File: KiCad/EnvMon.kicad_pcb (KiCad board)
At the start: 2 copper layers, 44.5 x 37 mm, 33 parts, among them J1 USB-C, J2 DC, J3 GPIO, M1 SCD30-4pin, M2 OLED1.5-RGB, U1 LMR16006+FB, U2 FT231XQ, U3 ESP32-WROOM-32

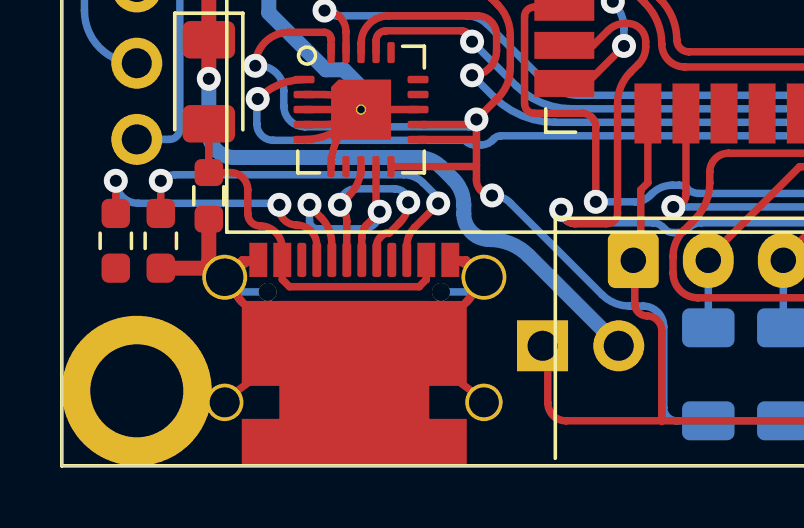
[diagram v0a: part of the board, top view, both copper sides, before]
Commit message: Notes
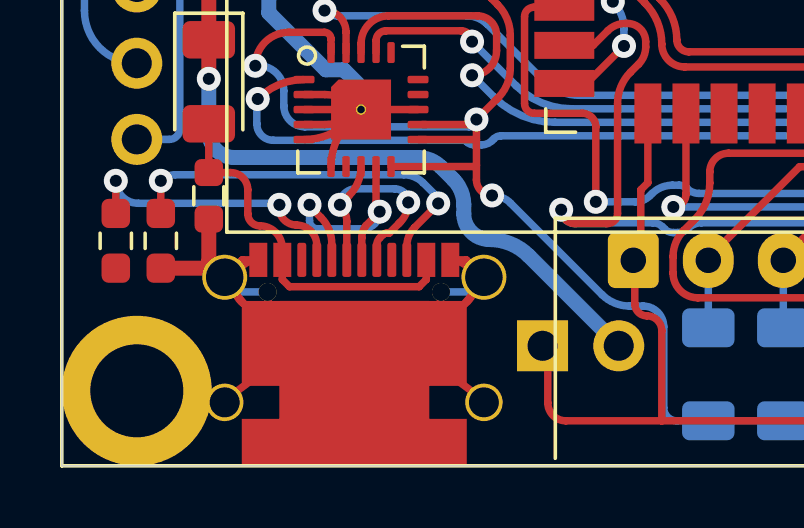
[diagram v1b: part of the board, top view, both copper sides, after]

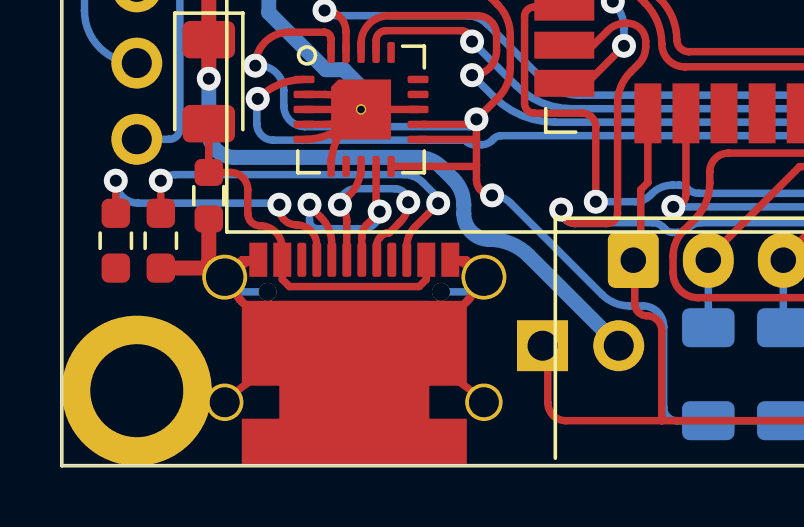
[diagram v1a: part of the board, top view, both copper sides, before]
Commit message: Resitors
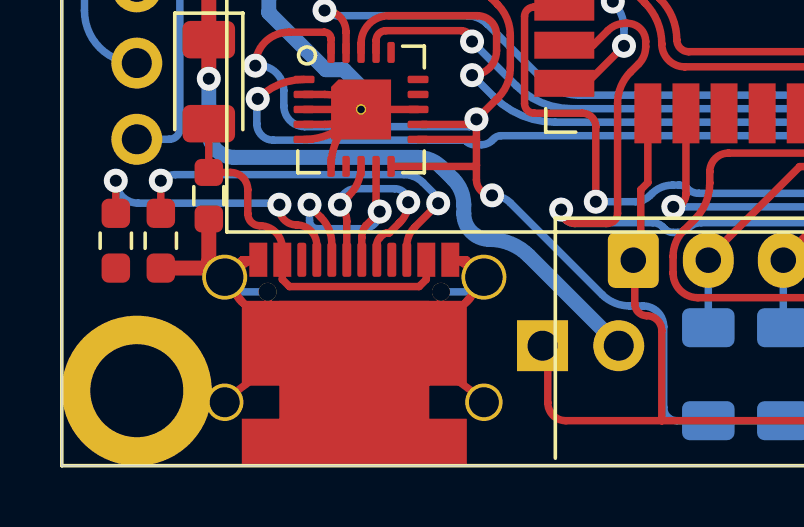
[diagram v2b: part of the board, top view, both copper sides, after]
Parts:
- R1: value 10M 1% or 0R -> 100k 1% or 0R
- R2: value 3M 1% or NF -> 30k 1% or NF
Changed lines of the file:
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@@
       (primitives
     (gr_arc (start 2.89 -3.045) (mid 0 -0.155) (end -2.89 -3.045) (width 0.25))
-    (gr_arc (start 4.294753 -3.49127) (mid -0.016568 -1.026234) (end -4.311371 -3.519937) (width 0.25))
+    (gr_arc (start 4.294753 -3.49127) (mid -0.012228 -1.026222) (end -4.307036 -3.512417) (width 0.25))
     (gr_arc (start -3.2 -2.485) (mid -4.015 -3.3) (end -3.2 -4.115) (width 0.25))
     (gr_arc (start 3.2 -4.115) (mid 4.015 -3.3) (end 3.2 -2.485) (width 0.25))
@@
       (effects (font (size 0.5 0.5) (thickness 0.08)))
     )
-    (fp_text value "10M 1% or 0R" (at 0 0 90) (layer "F.Fab")
+    (fp_text value "100k 1% or 0R" (at 0 0 90) (layer "F.Fab")
       (effects (font (size 0.4 0.4) (thickness 0.08)))
     )
@@
       (effects (font (size 0.5 0.5) (thickness 0.08)))
     )
-    (fp_text value "3M 1% or NF" (at 0 0 90) (layer "F.Fab")
+    (fp_text value "30k 1% or NF" (at 0 0 90) (layer "F.Fab")
       (effects (font (size 0.4 0.4) (thickness 0.08)))
     )
